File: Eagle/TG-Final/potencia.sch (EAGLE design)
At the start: 28 parts, among them IC1 7812T, Q1 2N3055, T1 2N3904

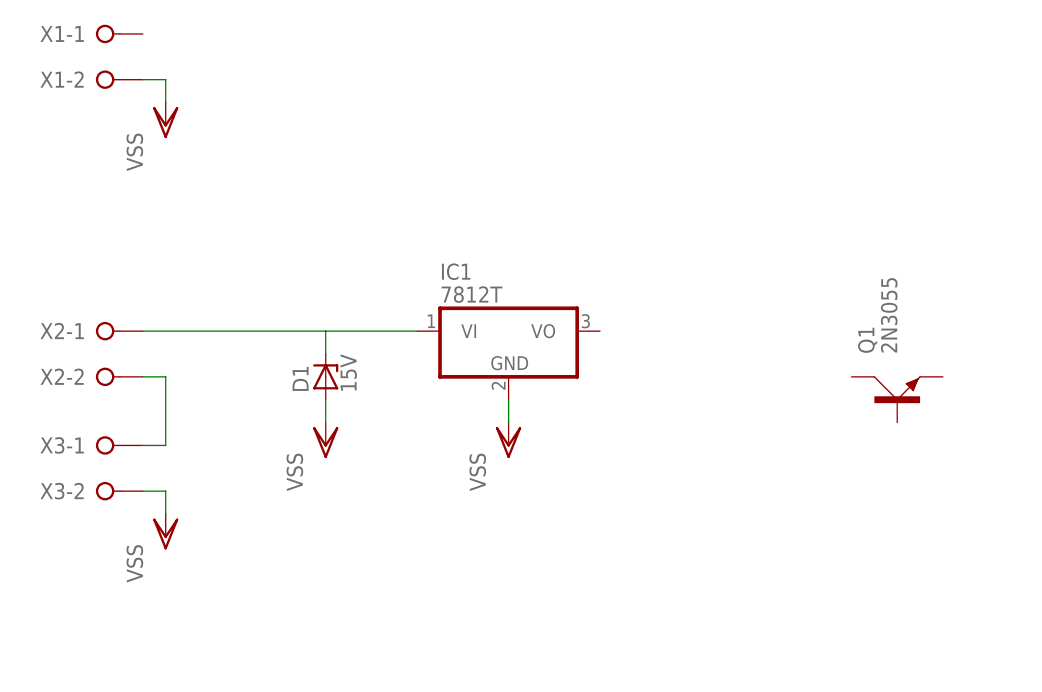
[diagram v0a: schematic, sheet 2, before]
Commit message: Esquematicos de Alimentación
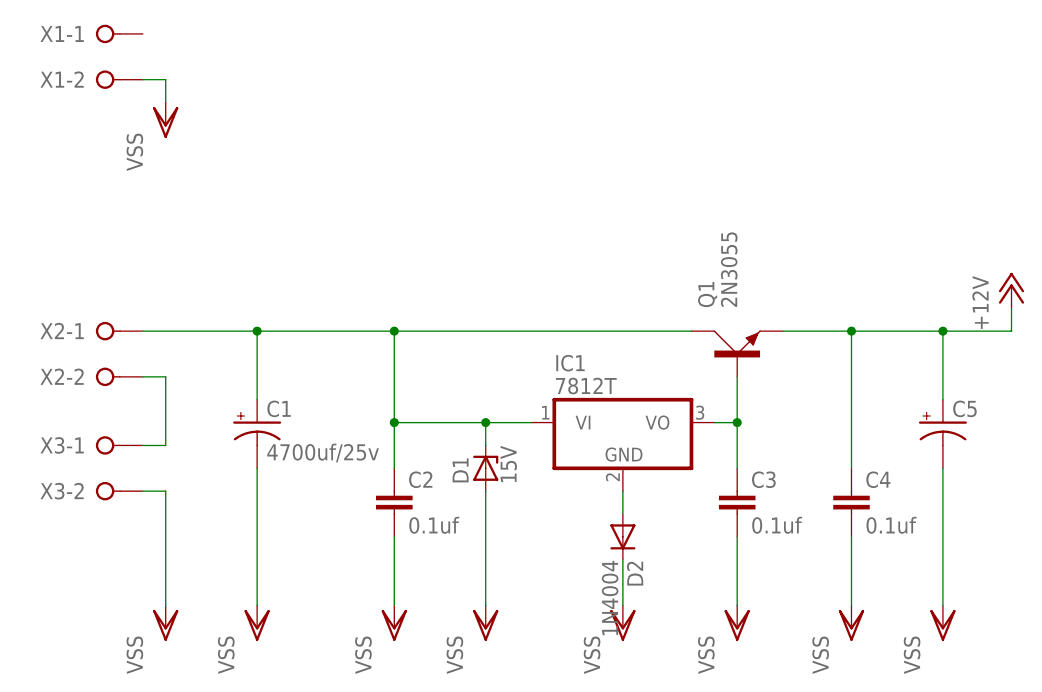
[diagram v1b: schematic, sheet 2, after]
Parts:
- added C1: 4700uf/25v, rcl:CPOL-USE10-30
- added C2, C3, C4: 0.1uf, rcl:C-EU050-024X044
- added C5: (no value), rcl:CPOL-USE2.5-6
- added D2: 1N4004, adafruit:1N4004
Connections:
- new net +12V: C4.1, C5.+, Q1.E
- new net N$22: C3.1, IC1.VO, Q1.B
- new net N$24: D2.A, IC1.GND
- net N$21: now also C1.+, C2.1, Q1.C
- net VSS: now also C1.-, C2.2, C3.2, C4.2, C5.-, D2.C; no longer IC1.GND
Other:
- moved on the sheet: D1, IC1, Q1
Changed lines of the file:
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@@
 <setting verticaltext="up"/>
 </settings>
-<grid distance="0.1" unitdist="inch" unit="inch" style="lines" multiple="1" display="no" altdistance="0.01" altunitdist="inch" altunit="inch"/>
+<grid distance="0.1" unitdist="inch" unit="inch" style="lines" multiple="1" display="yes" altdistance="0.01" altunitdist="inch" altunit="inch"/>
 <layers>
 <layer number="1" name="Top" color="4" fill="1" visible="no" active="no"/>
@@
 <part name="D1" library="diode" deviceset="ZENER-DIODE" device="F126-10" value="15V"/>
 <part name="VSS10" library="supply1" deviceset="VSS" device=""/>
+<part name="C1" library="rcl" deviceset="CPOL-US" device="E10-30" value="4700uf/25v"/>
+<part name="VSS12" library="supply1" deviceset="VSS" device=""/>
+<part name="C2" library="rcl" deviceset="C-EU" device="050-024X044" value="0.1uf"/>
 <part name="VSS11" library="supply1" deviceset="VSS" device=""/>
+<part name="D2" library="adafruit" deviceset="1N4004" device=""/>
+<part name="VSS13" library="supply1" deviceset="VSS" device=""/>
+<part name="C3" library="rcl" deviceset="C-EU" device="050-024X044" value="0.1uf"/>
+<part name="VSS14" library="supply1" deviceset="VSS" device=""/>
+<part name="C4" library="rcl" deviceset="C-EU" device="050-024X044" value="0.1uf"/>
+<part name="VSS15" library="supply1" deviceset="VSS" device=""/>
+<part name="C5" library="rcl" deviceset="CPOL-US" device="E2.5-6"/>
+<part name="VSS16" library="supply1" deviceset="VSS" device=""/>
+<part name="P+1" library="supply1" deviceset="+12V" device=""/>
 </parts>
 <sheets>
@@
 <instance part="X3" gate="-1" x="27.94" y="30.48"/>
 <instance part="X3" gate="-2" x="27.94" y="25.4"/>
-<instance part="VSS8" gate="G$1" x="35.56" y="20.32"/>
+<instance part="VSS8" gate="G$1" x="35.56" y="10.16"/>
 <instance part="VSS9" gate="G$1" x="35.56" y="66.04"/>
-<instance part="Q1" gate="A" x="116.84" y="35.56" rot="R90"/>
-<instance part="IC1" gate="A1" x="73.66" y="43.18"/>
-<instance part="D1" gate="G$1" x="53.34" y="38.1" rot="R90"/>
-<instance part="VSS10" gate="G$1" x="53.34" y="30.48"/>
-<instance part="VSS11" gate="G$1" x="73.66" y="30.48"/>
+<instance part="Q1" gate="A" x="99.06" y="40.64" rot="R90"/>
+<instance part="IC1" gate="A1" x="86.36" y="33.02"/>
+<instance part="D1" gate="G$1" x="71.12" y="27.94" rot="R90"/>
+<instance part="VSS10" gate="G$1" x="71.12" y="10.16"/>
+<instance part="C1" gate="G$1" x="45.72" y="33.02"/>
+<instance part="VSS12" gate="G$1" x="45.72" y="10.16"/>
+<instance part="C2" gate="G$1" x="60.96" y="25.4"/>
+<instance part="VSS11" gate="G$1" x="60.96" y="10.16"/>
+<instance part="D2" gate="1" x="86.36" y="20.32" rot="R270"/>
+<instance part="VSS13" gate="G$1" x="86.36" y="10.16"/>
+<instance part="C3" gate="G$1" x="99.06" y="25.4"/>
+<instance part="VSS14" gate="G$1" x="99.06" y="10.16"/>
+<instance part="C4" gate="G$1" x="111.76" y="25.4"/>
+<instance part="VSS15" gate="G$1" x="111.76" y="10.16"/>
+<instance part="C5" gate="G$1" x="121.92" y="33.02"/>
+<instance part="VSS16" gate="G$1" x="121.92" y="10.16"/>
+<instance part="P+1" gate="1" x="129.54" y="48.26"/>
 </instances>
 <busses>
@@
 <pinref part="VSS8" gate="G$1" pin="VSS"/>
 <wire x1="33.02" y1="25.4" x2="35.56" y2="25.4" width="0.1524" layer="91"/>
-<wire x1="35.56" y1="25.4" x2="35.56" y2="22.86" width="0.1524" layer="91"/>
+<wire x1="35.56" y1="25.4" x2="35.56" y2="12.7" width="0.1524" layer="91"/>
 </segment>
 <segment>
@@
 <pinref part="D1" gate="G$1" pin="A"/>
 <pinref part="VSS10" gate="G$1" pin="VSS"/>
-<wire x1="53.34" y1="35.56" x2="53.34" y2="33.02" width="0.1524" layer="91"/>
-</segment>
-<segment>
+<wire x1="71.12" y1="25.4" x2="71.12" y2="12.7" width="0.1524" layer="91"/>
+</segment>
+<segment>
+<pinref part="VSS12" gate="G$1" pin="VSS"/>
+<pinref part="C1" gate="G$1" pin="-"/>
+<wire x1="45.72" y1="12.7" x2="45.72" y2="27.94" width="0.1524" layer="91"/>
+</segment>
+<segment>
+<pinref part="VSS11" gate="G$1" pin="VSS"/>
+<pinref part="C2" gate="G$1" pin="2"/>
+<wire x1="60.96" y1="12.7" x2="60.96" y2="20.32" width="0.1524" layer="91"/>
+</segment>
+<segment>
+<pinref part="VSS13" gate="G$1" pin="VSS"/>
+<pinref part="D2" gate="1" pin="C"/>
+<wire x1="86.36" y1="12.7" x2="86.36" y2="17.78" width="0.1524" layer="91"/>
+</segment>
+<segment>
+<pinref part="VSS14" gate="G$1" pin="VSS"/>
+<pinref part="C3" gate="G$1" pin="2"/>
+<wire x1="99.06" y1="12.7" x2="99.06" y2="20.32" width="0.1524" layer="91"/>
+</segment>
+<segment>
+<pinref part="VSS15" gate="G$1" pin="VSS"/>
+<pinref part="C4" gate="G$1" pin="2"/>
+<wire x1="111.76" y1="12.7" x2="111.76" y2="20.32" width="0.1524" layer="91"/>
+</segment>
+<segment>
+<pinref part="C5" gate="G$1" pin="-"/>
+<pinref part="VSS16" gate="G$1" pin="VSS"/>
+<wire x1="121.92" y1="27.94" x2="121.92" y2="12.7" width="0.1524" layer="91"/>
+</segment>
+</net>
+<net name="N$21" class="0">
+<segment>
+<pinref part="X2" gate="-1" pin="KL"/>
+<wire x1="33.02" y1="43.18" x2="45.72" y2="43.18" width="0.1524" layer="91"/>
+<pinref part="C1" gate="G$1" pin="+"/>
+<wire x1="45.72" y1="35.56" x2="45.72" y2="43.18" width="0.1524" layer="91"/>
+<pinref part="Q1" gate="A" pin="C"/>
+<wire x1="93.98" y1="43.18" x2="60.96" y2="43.18" width="0.1524" layer="91"/>
+<pinref part="C2" gate="G$1" pin="1"/>
+<wire x1="60.96" y1="43.18" x2="45.72" y2="43.18" width="0.1524" layer="91"/>
+<wire x1="60.96" y1="27.94" x2="60.96" y2="33.02" width="0.1524" layer="91"/>
+<pinref part="IC1" gate="A1" pin="VI"/>
+<wire x1="60.96" y1="33.02" x2="60.96" y2="43.18" width="0.1524" layer="91"/>
+<wire x1="76.2" y1="33.02" x2="71.12" y2="33.02" width="0.1524" layer="91"/>
+<wire x1="71.12" y1="33.02" x2="60.96" y2="33.02" width="0.1524" layer="91"/>
+<pinref part="D1" gate="G$1" pin="C"/>
+<wire x1="71.12" y1="30.48" x2="71.12" y2="33.02" width="0.1524" layer="91"/>
+<junction x="71.12" y="33.02"/>
+<junction x="60.96" y="33.02"/>
+<junction x="60.96" y="43.18"/>
+<junction x="45.72" y="43.18"/>
+</segment>
+</net>
+<net name="N$22" class="0">
+<segment>
+<pinref part="IC1" gate="A1" pin="VO"/>
+<pinref part="Q1" gate="A" pin="B"/>
+<wire x1="96.52" y1="33.02" x2="99.06" y2="33.02" width="0.1524" layer="91"/>
+<wire x1="99.06" y1="33.02" x2="99.06" y2="38.1" width="0.1524" layer="91"/>
+<pinref part="C3" gate="G$1" pin="1"/>
+<wire x1="99.06" y1="27.94" x2="99.06" y2="33.02" width="0.1524" layer="91"/>
+<junction x="99.06" y="33.02"/>
+</segment>
+</net>
+<net name="N$24" class="0">
+<segment>
+<pinref part="D2" gate="1" pin="A"/>
 <pinref part="IC1" gate="A1" pin="GND"/>
-<pinref part="VSS11" gate="G$1" pin="VSS"/>
-<wire x1="73.66" y1="35.56" x2="73.66" y2="33.02" width="0.1524" layer="91"/>
-</segment>
-</net>
-<net name="N$21" class="0">
-<segment>
-<pinref part="IC1" gate="A1" pin="VI"/>
-<pinref part="D1" gate="G$1" pin="C"/>
-<wire x1="63.5" y1="43.18" x2="53.34" y2="43.18" width="0.1524" layer="91"/>
-<wire x1="53.34" y1="43.18" x2="53.34" y2="40.64" width="0.1524" layer="91"/>
-<pinref part="X2" gate="-1" pin="KL"/>
-<wire x1="33.02" y1="43.18" x2="53.34" y2="43.18" width="0.1524" layer="91"/>
-</segment>
-</net>
+<wire x1="86.36" y1="22.86" x2="86.36" y2="25.4" width="0.1524" layer="91"/>
+</segment>
+</net>
+<net name="+12V" class="0">
+<segment>
+<pinref part="P+1" gate="1" pin="+12V"/>
+<wire x1="129.54" y1="45.72" x2="129.54" y2="43.18" width="0.1524" layer="91"/>
+<pinref part="C4" gate="G$1" pin="1"/>
+<wire x1="111.76" y1="27.94" x2="111.76" y2="43.18" width="0.1524" layer="91"/>
+<pinref part="Q1" gate="A" pin="E"/>
+<wire x1="111.76" y1="43.18" x2="104.14" y2="43.18" width="0.1524" layer="91"/>
+<pinref part="C5" gate="G$1" pin="+"/>
+<wire x1="121.92" y1="35.56" x2="121.92" y2="43.18" width="0.1524" layer="91"/>
+<wire x1="121.92" y1="43.18" x2="111.76" y2="43.18" width="0.1524" layer="91"/>
+<wire x1="129.54" y1="43.18" x2="121.92" y2="43.18" width="0.1524" layer="91"/>
+<junction x="111.76" y="43.18"/>
+<junction x="121.92" y="43.18"/>
+</segment>
+</net>
